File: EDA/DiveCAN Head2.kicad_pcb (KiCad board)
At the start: 4 copper layers, 123 x 26 mm, 120 parts, among them J1 Analog Connection, J2 Digital Connection, J3 Conn_01x06_Pin, J4 Micro_SD_Card, SW1 RST, SW2 RST, U1 ADS1115IDGS, U10 TPS63000, U2 ADS1115IDGS, U3 STM32L431RCTx, U4 TPS2115, U5 TCAN33X, U6 TPS2115, U7 TPS2115, U8 TPS63000, U9 TPS63000, Y1 8MHz

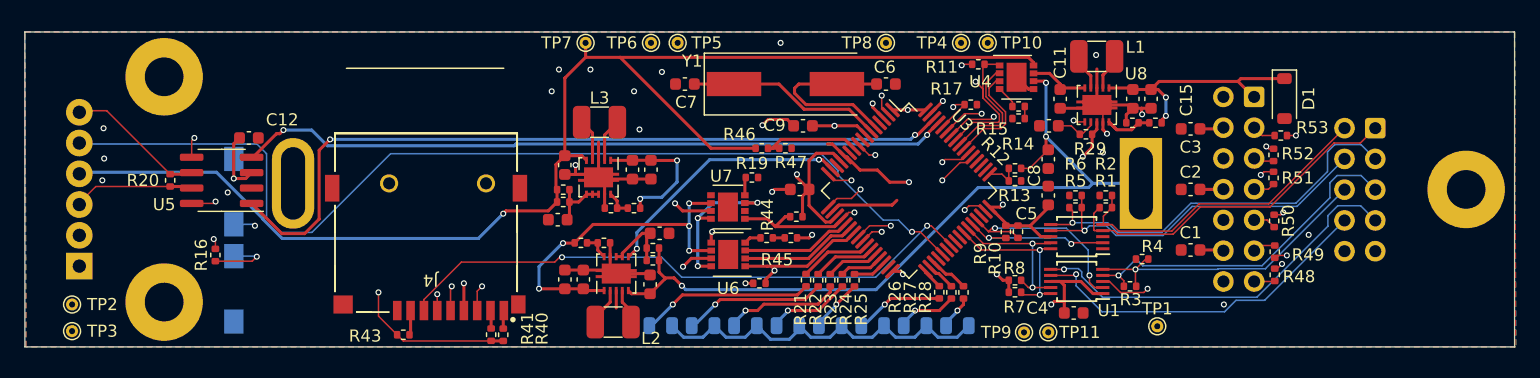
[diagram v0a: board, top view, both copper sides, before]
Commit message: Draft Rev2 PCB
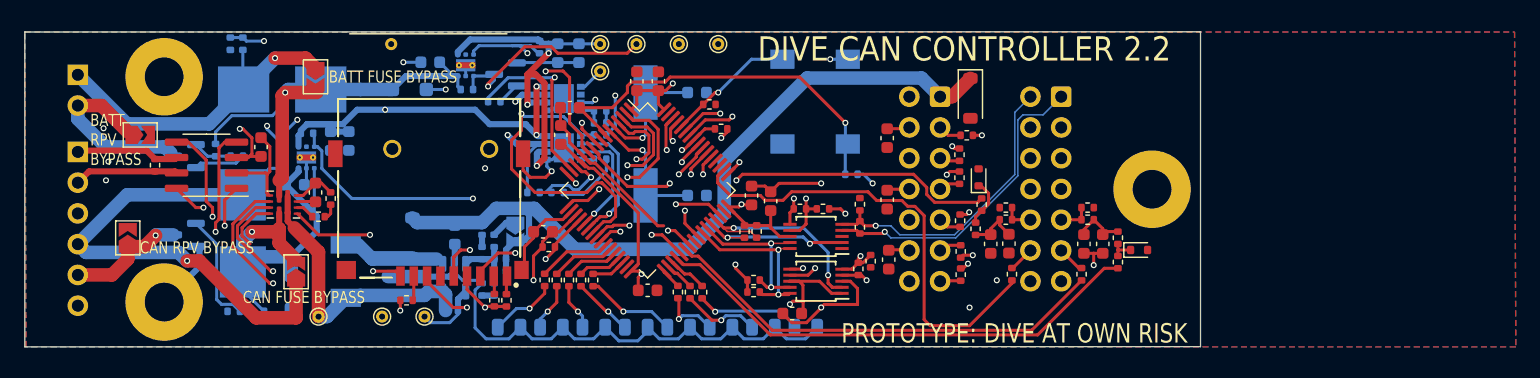
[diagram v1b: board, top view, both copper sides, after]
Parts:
- removed the C10 at (142.5, 84.5)
- removed the C11 at (164.0, 77.0)
- removed the J3 at (83.0, 90.8)
- removed L2, L3: 2.2u, Library:L_4x4
- removed the R1 at (167.8, 86.0)
- removed the R12 at (160.2, 82.8)
- removed the R13 at (160.2, 83.8)
- removed the R29 at (166.1, 79.9)
- removed the R30 at (171.8, 79.0)
- removed the R31 at (169.9, 79.0)
- removed the R32 at (130.4, 90.4)
- removed the R33 at (130.4, 89.3)
- removed the R34 at (124.4, 88.9)
- removed the R35 at (126.3, 88.9)
- removed the R36 at (123.0, 84.5)
- removed the R37 at (123.0, 85.5)
- removed the R38 at (128.8, 86.0)
- removed the R39 at (126.9, 86.0)
- removed the R4 at (170.8, 90.2)
- removed the R42 at (141.8, 88.5)
- removed the TP1 at (172.0, 95.8)
- removed TP11: VCC_STAT, TestPoint:TestPoint_THTPad_D1.0mm_Drill0.5mm
- removed TP7: CAN_PWR, TestPoint:TestPoint_THTPad_D1.0mm_Drill0.5mm
- removed the U1 at (165.3, 92.1)
- removed the U2 at (165.3, 88.4)
- added C24: 10u, Capacitor_SMD:C_0603_1608Metric, B.Cu at (114.0, 88.2)
- added C25: 100n, Capacitor_SMD:C_0603_1608Metric, F.Cu at (140.1, 85.5)
- added C26: 100n, Capacitor_SMD:C_0603_1608Metric, F.Cu at (141.9, 94.7)
- added C27: 100n, Capacitor_SMD:C_0603_1608Metric, F.Cu at (102.5, 84.8)
- added C28: 100n, Capacitor_SMD:C_0603_1608Metric, F.Cu at (130.8, 75.6)
- added C29: 100n, Capacitor_SMD:C_0603_1608Metric, F.Cu at (138.5, 85.0)
- added C30: 100n, Capacitor_SMD:C_0603_1608Metric, F.Cu at (129.9, 92.8)
- added C31: 100n, Capacitor_SMD:C_0603_1608Metric, F.Cu at (121.3, 88.0)
- added C32: 100n, Capacitor_SMD:C_0603_1608Metric, F.Cu at (129.0, 75.6)
- added C6: 100n, Capacitor_SMD:C_0603_1608Metric, F.Cu at (165.9, 89.0)
- added C7: 100n, Capacitor_SMD:C_0603_1608Metric, F.Cu at (159.8, 89.0)
- added D12: MBR0520, Diode_SMD:D_SOD-123, B.Cu at (110.5, 88.5)
- added D13: SMF12A, Diode_SMD:D_SOD-123F, B.Cu at (110.2, 76.2)
- added D14: SMF12A, Diode_SMD:D_SOD-123F, B.Cu at (100.5, 93.0)
- added D2: BZX584C2V4, Diode_SMD:D_SOD-523, F.Cu at (157.2, 83.5)
- added D3: BZX584C2V4, Diode_SMD:D_SOD-523, F.Cu at (170.5, 89.5)
- added F1: 2A, Fuse:Fuseholder_Littelfuse_Nano2_154x, B.Cu at (99.8, 76.2)
- added F2: 2A, Fuse:Fuseholder_Littelfuse_Nano2_154x, B.Cu at (96.5, 88.1)
- added G***: LOGO, LOGO, B.Cu at (134.1, 91.1)
- added J2: Analog Connection, Connector_IDC:IDC-Header_2x07_P2.54mm_Vertical, B.Cu at (164.1, 76.8)
- added JP1: 6V_OUT, Jumper:SolderJumper-2_P1.3mm_Open_TrianglePad1.0x1.5mm, B.Cu at (119.0, 88.0)
- added JP2: BATT_FUSE_BYPASS, Jumper:SolderJumper-2_P1.3mm_Open_TrianglePad1.0x1.5mm, F.Cu at (102.5, 75.2)
- added JP3: CAN_FUSE_BYPASS, Jumper:SolderJumper-2_P1.3mm_Open_TrianglePad1.0x1.5mm, F.Cu at (100.9, 91.3)
- added JP4: BATT_RVP_BYPASS, Jumper:SolderJumper-2_P1.3mm_Open_TrianglePad1.0x1.5mm, F.Cu at (88.0, 80.0)
- added JP5: CAN_RVP_BYPASS, Jumper:SolderJumper-2_P1.3mm_Open_TrianglePad1.0x1.5mm, F.Cu at (87.0, 88.5)
- added Q1: SI2302, Package_TO_SOT_SMD:SOT-23, B.Cu at (91.7, 81.8)
- added Q2: SI2302, Package_TO_SOT_SMD:SOT-23, B.Cu at (91.7, 88.2)
- added Q3: 2N7000, Package_TO_SOT_SMD:SOT-23, B.Cu at (118.2, 75.0)
- added R16: 10k, Resistor_SMD:R_0402_1005Metric, F.Cu at (157.5, 85.8)
- added R17: 10k, Resistor_SMD:R_0402_1005Metric, F.Cu at (168.8, 90.5)
- added R18: 10k, Resistor_SMD:R_0402_1005Metric, F.Cu at (157.0, 87.8)
- added R20: 22k, Resistor_SMD:R_0402_1005Metric, F.Cu at (159.5, 87.0)
- added R21: 1k, Resistor_SMD:R_0402_1005Metric, F.Cu at (159.5, 86.0)
- added R22: 22k, Resistor_SMD:R_0402_1005Metric, F.Cu at (166.2, 87.0)
- added R23: 1k, Resistor_SMD:R_0402_1005Metric, F.Cu at (166.2, 86.0)
- added R24: 200, Resistor_SMD:R_0402_1005Metric, F.Cu at (165.8, 91.5)
- added R25: 200, Resistor_SMD:R_0402_1005Metric, F.Cu at (160.0, 91.5)
- added R45: 10k, Resistor_SMD:R_0402_1005Metric, B.Cu at (121.0, 72.8)
- added R48: 1.2k, Resistor_SMD:R_0402_1005Metric, B.Cu at (116.2, 92.8)
- added R49: 15k, Resistor_SMD:R_0402_1005Metric, B.Cu at (116.2, 89.8)
- added R50: 100k, Resistor_SMD:R_0402_1005Metric, B.Cu at (117.2, 88.8)
- added R51: 100k, Resistor_SMD:R_0402_1005Metric, B.Cu at (116.2, 87.8)
- added R52: 22k, Resistor_SMD:R_0402_1005Metric, F.Cu at (147.4, 87.6)
- added R53: 200, Resistor_SMD:R_0402_1005Metric, F.Cu at (147.4, 85.7)
- added R54: 22k, Resistor_SMD:R_0402_1005Metric, F.Cu at (147.3, 91.1)
- added R55: 200, Resistor_SMD:R_0402_1005Metric, F.Cu at (148.3, 90.4)
- added R56: 22k, Resistor_SMD:R_0402_1005Metric, F.Cu at (142.5, 86.1)
- added R57: 200, Resistor_SMD:R_0402_1005Metric, F.Cu at (144.4, 86.1)
- added R58: 10k, Resistor_SMD:R_0402_1005Metric, B.Cu at (94.2, 81.2)
- added R59: 10k, Resistor_SMD:R_0402_1005Metric, B.Cu at (97.8, 94.6)
- added R60: 100k, Resistor_SMD:R_0402_1005Metric, B.Cu at (96.0, 81.8)
- added R61: 100k, Resistor_SMD:R_0402_1005Metric, B.Cu at (95.8, 94.6)
- added R62: 10k, Resistor_SMD:R_0402_1005Metric, B.Cu at (115.0, 76.2)
- added R63: 800, Resistor_SMD:R_0402_1005Metric, B.Cu at (117.3, 77.2)
- added R65: 10k, Resistor_SMD:R_0402_1005Metric, B.Cu at (126.0, 78.0)
- added R66: 10k, Resistor_SMD:R_0402_1005Metric, B.Cu at (126.0, 79.0)
- added R67: 2.2k, Resistor_SMD:R_0402_1005Metric, B.Cu at (126.0, 82.0)
- added R69: 100k, Resistor_SMD:R_0402_1005Metric, F.Cu at (102.8, 86.8)
- added R70: 10k, Resistor_SMD:R_0402_1005Metric, F.Cu at (103.8, 85.2)
- added TP4: BAT_REG, TestPoint:TestPoint_THTPad_D1.0mm_Drill0.5mm, F.Cu at (126.0, 72.5)
- added U3: TPS7A2533DRVR, Package_SON:WSON-6-1EP_2x2mm_P0.65mm_EP1x1.6mm_ThermalVias, B.Cu at (101.8, 81.9)
- added U5: LMR62014XMF, Package_TO_SOT_SMD:SOT-23-5, B.Cu at (114.0, 91.8)
- BT1: footprint Library:BatteryHolder_MPD_BH-18650-PC2 -> Connector_PinHeader_2.54mm:PinHeader_1x02_P2.54mm_Horizontal
- C1: renamed from C6; moved to B.Cu
- C13, C16: value 100n -> 10u; moved to B.Cu
- C14, C17, C21: value 10u -> 100n; moved to B.Cu
- C15, C18, C19, C20, Y1: moved to B.Cu
- C2: renamed from C7; moved to B.Cu
- C22, C23: value 10u -> 100p; footprint Capacitor_SMD:C_0603_1608Metric -> Capacitor_SMD:C_0402_1005Metric; moved to B.Cu
- C8: value 10u -> 100n
- J1: value Analog Connection -> Micro_SD_Card_Det1; footprint Connector_IDC:IDC-Header_2x05_P2.54mm_Vertical -> Library:CONN9_0185-02_GSW; moved to F.Cu
- J4: value Micro_SD_Card -> CAN Connection; footprint Library:CONN9_0185-02_GSW -> Connector_PinHeader_2.54mm:PinHeader_1x06_P2.54mm_Horizontal; moved to B.Cu
- L1: value 2.2u -> 10u; footprint Library:L_4x4 -> Library:L_SunItech_SLO0530H; moved to B.Cu
- R1: renamed from R16; moved to B.Cu
- R13: renamed from R45; moved to B.Cu
- R14: value 200 -> 100k; moved to B.Cu
- R15, R44: value 200 -> 10k; moved to B.Cu
- R19: value 800 -> 10k
- R2: value 200 -> 12k; moved to B.Cu
- R3, R47: value 10k -> 12k; moved to B.Cu
- R36: renamed from R21; value 10k -> 5.1k
- R37: renamed from R22; value 10k -> 5.1k
- R38: renamed from R23; value 10k -> 5.1k
- R39: renamed from R24; value 10k -> 5.1k
- R40: renamed from R25; value 10k -> 5.1k
- R41: renamed from R26; value 10k -> 5.1k
- R42: renamed from R27; value 10k -> 5.1k
- R43: renamed from R28; value 10k -> 5.1k
- R46: value 10k -> 100k; moved to B.Cu
- R5: value 10k -> 75k; moved to B.Cu
- R6: value 200 -> 75k; moved to B.Cu
- TP10: value SOL_STAT -> SOLENOID_PWR
- TP2: value VCC -> BAT_EN
- TP3: value VBUS -> CAN_REG; moved to B.Cu
- TP5: value BAT_REG -> VCC_STAT
- TP6: value CAN_REG -> BUS_STAT
- TP8: value BAT_EN -> VCC
- TP9: value BUS_STAT -> VBUS
- U10: value TPS63000 -> TPS2121; footprint Package_SON:Texas_DRC0010J -> Package_DFN_QFN:Texas_VQFN-HR-12_2x2.5mm_P0.5mm
- U4: value TPS2115 -> TPS7A2533DRVR; footprint Library:VSON-8_3.3x3.3mm_P0.65mm_NexFET -> Package_SON:WSON-6-1EP_2x2mm_P0.65mm_EP1x1.6mm_ThermalVias; moved to B.Cu
- U6, U7: value TPS2115 -> ADS1115IDGS; footprint Library:VSON-8_3.3x3.3mm_P0.65mm_NexFET -> Package_SO:TSSOP-10_3x3mm_P0.5mm
- U8, U9: value TPS63000 -> TPS2115; footprint Package_SON:Texas_DRC0010J -> Library:VSON-8_3.3x3.3mm_P0.65mm_NexFET; moved to B.Cu
- moved J1 78.3 mm to (111.9, 84.8)
- moved R2 73.4 mm to (95.5, 72.5), turned to -90 degrees
- moved R3 71.1 mm to (99.8, 80.2), turned to 90 degrees
- moved R6 69.9 mm to (96.5, 72.5), turned to 90 degrees
- moved C14 66.3 mm to (103.8, 80.5)
- moved C15 66.3 mm to (105.2, 80.5)
- moved R5 65.6 mm to (99.8, 82.2), turned to 90 degrees
- moved L1 64.5 mm to (105.0, 91.2), turned to 90 degrees
- moved C13 62.4 mm to (100.8, 84.1)
- moved TP10 59.7 mm to (102.8, 95.0), turned to 0 degrees
- moved BT1 53.5 mm to (82.9, 75.0)
- moved TP9 53.0 mm to (108.0, 95.0), turned to 0 degrees
- moved R1 52.9 mm to (146.8, 83.2), turned to 0 degrees
- moved TP2 51.3 mm to (129.0, 72.5), turned to 0 degrees
- moved TP1 49.7 mm to (111.5, 95.0)
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- renumbered C1 to C10, C2 to C11, C3 to C12, C9 to C3, C12 to C9, D8 to D10, D9 to D11, D2 to D4, D3 to D5, D4 to D6, D5 to D7, D6 to D8, D7 to D9, H4 to H3, J2 to J3, R18 to R12, R48 to R26, R49 to R27, R50 to R28, R51 to R29, R52 to R30, R53 to R31, R43 to R32, R41 to R33, R40 to R34, R20 to R35, R17 to R4, TP4 to TP1, U3 to U1, U5 to U2
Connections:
- net Net-(U3-PB8) renamed /CAN_RX
- net Net-(U3-PB9) renamed /CAN_TX
- BT1 pad 2: GNDREF -> /Power Distribution/BATT_GND
- C13 pad 1: GNDREF -> /Power Distribution/CAN
- C13 pad 2: Net-(U8-PS/SYNC) -> GNDREF
- C14 pad 1: /SOL_OUT -> /Power Distribution/CAN_REGULATED
- C15 pad 1: /SOL_OUT -> /Power Distribution/CAN_REGULATED
- C16 pad 1: GNDREF -> /Power Distribution/BATTERY
- C16 pad 2: Net-(U9-PS/SYNC) -> GNDREF
- C17 pad 1: /BATTERY_REGULATED -> /Power Distribution/BATTERY_REGULATED
- C18 pad 1: /BATTERY_REGULATED -> /Power Distribution/BATTERY_REGULATED
- C19 pad 2: Net-(U10-EN) -> /Power Distribution/SOLENOID_PWR
- C20 pad 1: /CAN_REGULATED -> /Power Distribution/SOLENOID_PWR
- C21 pad 1: /CAN_REGULATED -> GNDREF
- C21 pad 2: GNDREF -> /Power Distribution/SOLENOID_PWR
- C22 pad 1: /BATTERY -> /SOL_OUT
- C22 pad 2: GNDREF -> Net-(U5-FB)
- C23 pad 1: /CAN_PWR -> /SOL_OUT
- C23 pad 2: GNDREF -> Net-(U5-FB)
- C4 pad 1: VCC -> GNDREF
- C4 pad 2: GNDREF -> VCC
- C5 pad 1: VCC -> GNDREF
- C5 pad 2: GNDREF -> Net-(C5-Pad2)
- C8 pad 2: /BATTERY -> Net-(C6-Pad2)
- J1 pad 1: /C1+ -> Net-(J1-DAT2)
- J1 pad 2: /C1- -> Net-(J1-DAT3/CD)
- J1 pad 3: /C2+ -> /SD_CMD
- J1 pad 4: /C2- -> VBUS
- J1 pad 5: /C3+ -> /SD_CLK
- J1 pad 6: /C3- -> GNDREF
- J1 pad 7: /AUX+ -> /SD_DAT0
- J1 pad 8: /AUX- -> Net-(J1-DAT1)
- J1 pad 9: VBUS -> /SD_DET
- J4 pad 1: Net-(J4-DAT2) -> Net-(J4-Pin_1)
- J4 pad 2: Net-(J4-DAT3/CD) -> Net-(J4-Pin_2)
- J4 pad 3: /SD_CMD -> /~{CAN_EN}
- J4 pad 4: VBUS -> /CAN_PWR
- J4 pad 5: /SD_CLK -> /CAN_GND
- J4 pad 6: GNDREF -> VBUS
- L1 pad 1: Net-(U8-L2) -> /Power Distribution/SOLENOID_PWR
- L1 pad 2: Net-(U8-L1) -> Net-(D12-A)
- R14 pad 1: GNDREF -> Net-(U1-PA0)
- R14 pad 2: Net-(R14-Pad2) -> VBUS
- R15 pad 1: Net-(R14-Pad2) -> GNDREF
- R15 pad 2: Net-(U4-I_LIM) -> Net-(U1-PA0)
- R19 pad 1: Net-(U7-I_LIM) -> Net-(C6-Pad2)
- R19 pad 2: GNDREF -> Net-(D3-K)
- R2 pad 1: /C1- -> Net-(U1-PC3)
- R3 pad 1: /C3+ -> Net-(U1-PC2)
- R3 pad 2: /C3- -> GNDREF
- R32 pad 1: Net-(J4-DAT1) -> Net-(J1-DAT1)
- R32 pad 2: VCC -> VBUS
- R33 pad 1: Net-(J4-DAT3/CD) -> Net-(J1-DAT3/CD)
- R33 pad 2: VCC -> VBUS
- R34 pad 1: Net-(J4-DAT2) -> Net-(J1-DAT2)
- R34 pad 2: VCC -> VBUS
- R35 pad 1: Net-(J3-Pin_3) (its old number) -> Net-(J4-Pin_2)
- R35 pad 2: Net-(J3-Pin_6) -> Net-(J4-Pin_1)
- R44 pad 1: Net-(R42-Pad2) -> /Power Distribution/CAN_REGULATED
- R44 pad 2: Net-(U6-I_LIM) -> /CAN_PG
- R46 pad 1: Net-(U3-PC2) -> /SOLENOID
- R46 pad 2: /CAN_PWR -> /Power Distribution/SOLENOID_PWR
- R47 pad 1: GNDREF -> Net-(U5-FB)
- R47 pad 2: Net-(U3-PC2) -> Net-(R47-Pad2)
- R5 pad 1: /C2+ -> /CAN_PWR
- R5 pad 2: /C2- -> Net-(U1-PC2)
- R6 pad 1: /C2- -> /BATTERY
- R6 pad 2: GNDREF -> Net-(U1-PC3)
- TP10 pad 1: /SOL_STAT -> /Power Distribution/SOLENOID_PWR
- TP2 pad 1: VCC -> /Power Distribution/BatteryConverter/ENABLE
- TP3 pad 1: VBUS -> /Power Distribution/CAN_REGULATED
- TP5 pad 1: /BATTERY_REGULATED -> /VCC_STAT
- TP6 pad 1: /CAN_REGULATED -> /BUS_STAT
- TP8 pad 1: /BATTERY_EN -> VCC
- TP9 pad 1: /BUS_STAT -> VBUS
- U1 pad 10: Net-(U3-PC2) -> Net-(U1-PC2)
- U1 pad 11: unconnected-(U3-PC3-Pad11) -> Net-(U1-PC3)
- U1 pad 14: unconnected-(U3-PA0-Pad14) -> Net-(U1-PA0)
- U1 pad 15: /BATTERY_EN -> /BATT_OFF
- U1 pad 2: /CAN_SILENT -> /~{CAN_EN}
- U1 pad 36: unconnected-(U3-PB15-Pad36) -> /PWM_2
- U1 pad 37: /~{CAN_EN} -> /SD_DET
- U1 pad 38: unconnected-(U3-PC7-Pad38) -> /GPIO_A
- U1 pad 4: unconnected-(U3-PC15-Pad4) -> /CAN_SILENT
- U1 pad 41: unconnected-(U3-PA8-Pad41) -> /PWM_1
- U1 pad 46: unconnected-(U3-PA13-Pad46) -> /CAN_PG
- U1 pad 49: Net-(U3-PA14) -> /BATT_PG
- U1 pad 50: unconnected-(U3-PA15-Pad50) -> /GPIO_B
- U1 pad 55: /SOL_SEL2 -> /SOL_DIS_BATT
- U1 pad 56: /SOL_SEL1 -> /SOL_DIS_CAN
- U10 pad 1: /CAN_REGULATED -> /Power Distribution/SOLENOID_PWR
- U10 pad 11: GNDREF -> Net-(U10-SS)
- U10 pad 2: Net-(U10-L2) -> /Power Distribution/BATTERY
- U10 pad 4: Net-(U10-L1) -> /SOL_DIS_BATT
- U10 pad 5: /CAN_PWR -> /SOL_DIS_CAN
- U10 pad 6: Net-(U10-EN) -> GNDREF
- U10 pad 7: Net-(U10-EN) -> /Power Distribution/CAN
- U10 pad 8: Net-(U10-EN) -> /Power Distribution/SOLENOID_PWR
- U10 pad 9: GNDREF -> /SOL_STAT
- U2 pad 6: Net-(J3-Pin_6) -> Net-(J4-Pin_1)
- U2 pad 7: Net-(J3-Pin_3) (its old number) -> Net-(J4-Pin_2)
- U4 pad 1: /SOL_STAT -> /Power Distribution/BATTERY_REGULATED
- U4 pad 2: /SOL_SEL1 -> unconnected-(U4-FB-Pad2)
- U4 pad 3: /SOL_SEL2 -> /BATT_PG
- U4 pad 4: Net-(U4-I_LIM) -> /Power Distribution/BatteryConverter/ENABLE
- U4 pad 6: /BATTERY -> /Power Distribution/BATTERY
- U4 pad 7: /Solenoid Driver/IN -> GNDREF
- U6 pad 1: /BUS_STAT -> GNDREF
- U6 pad 2: /BUS_SEL1 -> /ALRT_ADC1
- U6 pad 3: /BUS_SEL2 -> GNDREF
- U6 pad 4: Net-(U6-I_LIM) -> /C1+
- U6 pad 5: GNDREF -> /C1-
- U6 pad 6: /BATTERY_REGULATED -> /C2+
- U6 pad 7: VBUS -> /C2-
- U6 pad 8: /CAN_REGULATED -> VCC
- U7 pad 1: /VCC_STAT -> VCC
- U7 pad 2: GNDREF -> /ALRT_ADC2
- U7 pad 3: /CAN_REGULATED -> GNDREF
- U7 pad 4: Net-(U7-I_LIM) -> /C3+
- U7 pad 5: GNDREF -> /C3-
- U7 pad 6: /BATTERY_REGULATED -> /AUX+
- U7 pad 7: VCC -> /AUX-
- U7 pad 8: /CAN_REGULATED -> VCC
- U8 pad 1: /SOL_OUT -> /VCC_STAT
- U8 pad 2: Net-(U8-L2) -> GNDREF
- U8 pad 3: GNDREF -> /Power Distribution/CAN_REGULATED
- U8 pad 4: Net-(U8-L1) -> Net-(U8-I_LIM)
- U8 pad 5: /Solenoid Driver/IN -> GNDREF
- U8 pad 6: /SOLENOID -> /Power Distribution/BATTERY_REGULATED
- U8 pad 7: Net-(U8-PS/SYNC) -> VCC
- U8 pad 8: VCC -> /Power Distribution/CAN_REGULATED
- U9 pad 1: /BATTERY_REGULATED -> /BUS_STAT
- U9 pad 2: Net-(U9-L2) -> /BUS_SEL1
- U9 pad 3: GNDREF -> /BUS_SEL2
- U9 pad 5: /BATTERY -> GNDREF
- U9 pad 6: /BATTERY_EN -> /Power Distribution/BATTERY_REGULATED
- U9 pad 7: Net-(U9-PS/SYNC) -> VBUS
- U9 pad 8: Net-(U9-PS/SYNC) -> /Power Distribution/CAN_REGULATED
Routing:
- net /CAN_PWR: track 110.7 -> 43.1 mm
- net /BOOT: track 67.6 -> 10.7 mm, vias 2 -> 1
- net /SOL_DIS_BATT: track 0.00 -> 51.3 mm, vias 0 -> 2
- net GNDREF: track 97.4 -> 147.7 mm, vias 27 -> 13
- net /SOL_DIS_CAN: track 0.00 -> 48.6 mm, vias 0 -> 2
- net /BATTERY: track 74.9 -> 27.1 mm, vias 3 -> 1
- net /SOL_OUT: track 20.4 -> 68.1 mm, vias 2 -> 0
- net Net-(U1-PC2): track 0.00 -> 47.1 mm, vias 0 -> 3
- net /CAN_REGULATED: track 46.7 -> 0.00 mm, vias 5 -> 0
- net /Power Distribution/CAN_REGULATED: track 0.00 -> 44.8 mm, vias 0 -> 4
- net /BATTERY_REGULATED: track 42.5 -> 0.00 mm, vias 5 -> 0
- net /PWM_2: track 0.00 -> 41.3 mm
- net /Power Distribution/BATTERY: track 0.00 -> 38.0 mm, vias 0 -> 1
- net /GPIO_B: track 0.00 -> 37.8 mm
- net /CAN_PG: track 0.00 -> 37.7 mm, vias 0 -> 2
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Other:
- board size 123 x 26 mm -> 97.1 x 26 mm
- board text added: "#:"
- board text added: "13.3V MAX"
- board text added: "6V SOL OUT"
- board text added: "B+ B-"
- board text added: "BATT FUSE BYPASS"
- board text added: "BATT RPV BYPASS"
- board text added: "C1+ C2+ C3+ AUX+ DAC1 IO A VBUS"
- board text added: "C1- C2- C3- AUX- DAC1 IO B GND"
- board text added: "CAN FUSE BYPASS"
- board text added: "CAN RPV BYPASS"
- board text added: "CAN_L ENABLE PWR+ CAN_H PWR- VBUS"
- board text added: "DIVE CAN CONTROLLER 2.2"
- board text added: "PROTOTYPE! DIVE AT OWN RISK"
- board text removed: "1+ 2+ 3+ A+ V"
- board text removed: "1- 2- 3- A- G"
- board text removed: "CAN_L ENABLE CAN_PWR CAN_H GND VBUS"
- board text removed: "DIVE CAN CONTROLLER 2.1"
- board text removed: "TP1"
- board text removed: "TP10"
- board text removed: "TP11 TP9"
- board text removed: "TP2"
- board text removed: "TP3"
- board text removed: "TP4"
- board text removed: "TP5"
- board text removed: "TP6"
- board text removed: "TP7"
- board text removed: "TP8"

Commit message: Rev 2.2 fabrication tweaks
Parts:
- R26, R27, R28, R29, R30, R31, R63: value 800 -> 680
